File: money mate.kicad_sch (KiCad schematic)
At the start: 17 parts, among them SW1 SW_Push, SW2 SW_Push, SW3 SW_Push, SW4 RotaryEncoder_Switch, U1 MOUDLE-SEEEDUINO-XIAO

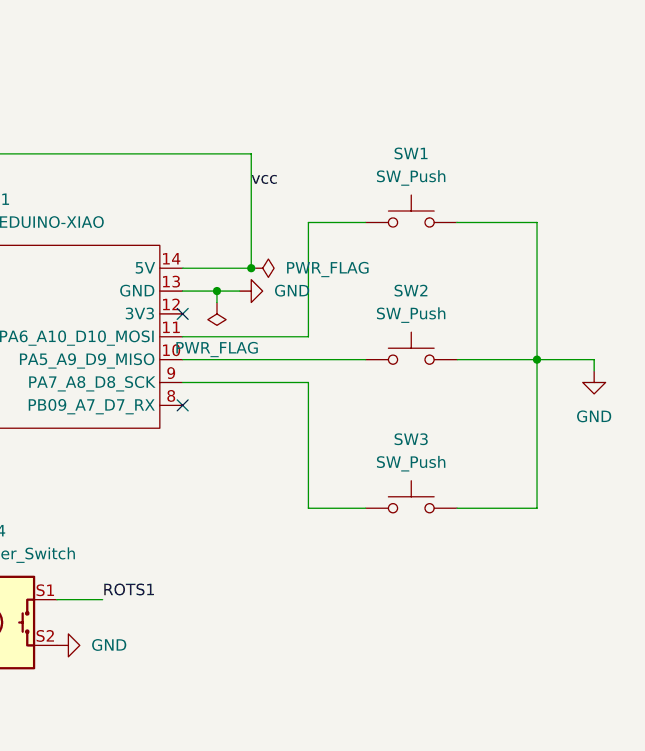
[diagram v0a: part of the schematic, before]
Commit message: pcb ready!!!!
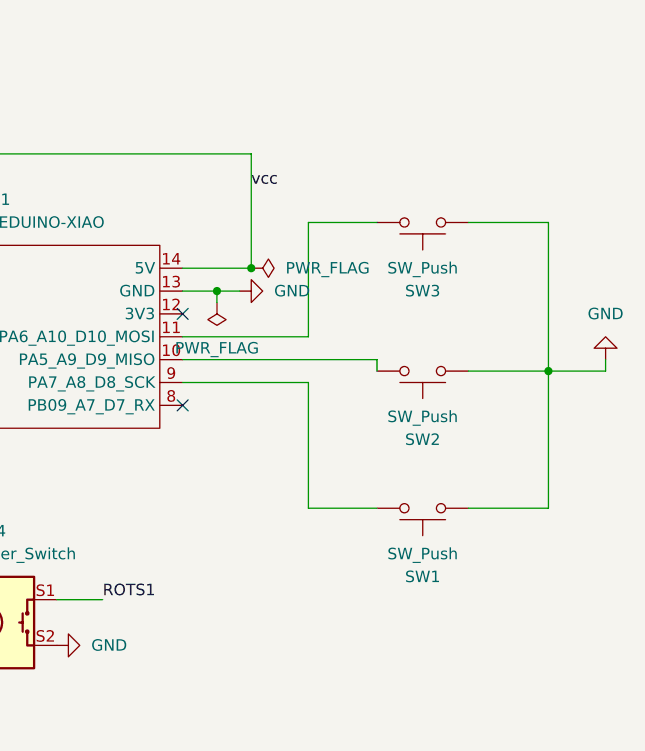
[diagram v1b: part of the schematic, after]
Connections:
- net at SW3.1: now also U1.11 (PA6_A10_D10_MOSI); no longer U1.9 (PA7_A8_D8_SCK)
- net at SW1.1: now also U1.9 (PA7_A8_D8_SCK); no longer U1.11 (PA6_A10_D10_MOSI)
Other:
- moved on the sheet: SW1, SW2, SW3
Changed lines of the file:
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@@
 	)
 	(junction
-		(at 233.68 86.36)
+		(at 234.95 87.63)
 		(diameter 0)
 		(color 0 0 0 0)
@@
 	(wire
 		(pts
+			(xy 215.9 87.63) (xy 215.9 86.36)
+		)
+		(stroke
+			(width 0)
+			(type default)
+		)
+	)
+	(wire
+		(pts
 			(xy 138.43 86.36) (xy 153.67 86.36)
 		)
@@
 	(wire
 		(pts
-			(xy 233.68 86.36) (xy 233.68 102.87)
+			(xy 234.95 87.63) (xy 234.95 71.12)
 		)
 		(stroke
@@
 	(wire
 		(pts
-			(xy 233.68 71.12) (xy 233.68 86.36)
+			(xy 234.95 102.87) (xy 234.95 87.63)
 		)
 		(stroke
@@
 	(wire
 		(pts
-			(xy 240.03 86.36) (xy 240.03 87.63)
+			(xy 241.3 87.63) (xy 241.3 86.36)
 		)
 		(stroke
@@
 	(wire
 		(pts
-			(xy 224.79 71.12) (xy 233.68 71.12)
+			(xy 226.06 102.87) (xy 234.95 102.87)
 		)
 		(stroke
@@
 	(wire
 		(pts
-			(xy 224.79 86.36) (xy 233.68 86.36)
+			(xy 226.06 87.63) (xy 234.95 87.63)
 		)
 		(stroke
@@
 	(wire
 		(pts
-			(xy 208.28 71.12) (xy 214.63 71.12)
+			(xy 208.28 71.12) (xy 215.9 71.12)
 		)
 		(stroke
@@
 	(wire
 		(pts
-			(xy 233.68 102.87) (xy 224.79 102.87)
+			(xy 234.95 71.12) (xy 226.06 71.12)
 		)
 		(stroke
@@
 	(wire
 		(pts
-			(xy 194.31 86.36) (xy 214.63 86.36)
+			(xy 194.31 86.36) (xy 215.9 86.36)
 		)
 		(stroke
@@
 	(wire
 		(pts
-			(xy 233.68 86.36) (xy 240.03 86.36)
+			(xy 234.95 87.63) (xy 241.3 87.63)
 		)
 		(stroke
@@
 	(wire
 		(pts
-			(xy 208.28 102.87) (xy 214.63 102.87)
+			(xy 208.28 102.87) (xy 215.9 102.87)
 		)
 		(stroke
@@
 	(symbol
 		(lib_id "power:GND")
-		(at 240.03 87.63 0)
+		(at 241.3 86.36 0)
+		(mirror x)
 		(unit 1)
 		(body_style 1)
@@
 		(fields_autoplaced yes)
 		(property "Reference" "#PWR02"
-			(at 240.03 93.98 0)
+			(at 241.3 80.01 0)
 			(hide yes)
 			(show_name no)
@@
 		)
 		(property "Value" "GND"
-			(at 240.03 92.71 0)
+			(at 241.3 81.28 0)
 			(show_name no)
 			(do_not_autoplace no)
@@
 		)
 		(property "Footprint" ""
-			(at 240.03 87.63 0)
+			(at 241.3 86.36 0)
 			(hide yes)
 			(show_name no)
@@
 		)
 		(property "Datasheet" ""
-			(at 240.03 87.63 0)
+			(at 241.3 86.36 0)
 			(hide yes)
 			(show_name no)
@@
 		)
 		(property "Description" "Power symbol creates a global label with name \"GND\" , ground"
-			(at 240.03 87.63 0)
+			(at 241.3 86.36 0)
 			(hide yes)
 			(show_name no)
@@
 	(symbol
 		(lib_id "Switch:SW_Push")
-		(at 219.71 102.87 0)
+		(at 220.98 71.12 0)
+		(mirror x)
 		(unit 1)
 		(body_style 1)
@@
 		(fields_autoplaced yes)
 		(property "Reference" "SW3"
-			(at 219.71 95.25 0)
+			(at 220.98 78.74 0)
 			(show_name no)
 			(do_not_autoplace no)
@@
 		)
 		(property "Value" "SW_Push"
-			(at 219.71 97.79 0)
+			(at 220.98 76.2 0)
 			(show_name no)
 			(do_not_autoplace no)
@@
 		)
 		(property "Footprint" "Button_Switch_Keyboard:SW_Cherry_MX_1.00u_PCB"
-			(at 219.71 97.79 0)
+			(at 220.98 76.2 0)
 			(hide yes)
 			(show_name no)
@@
 		)
 		(property "Datasheet" ""
-			(at 219.71 97.79 0)
+			(at 220.98 76.2 0)
 			(hide yes)
 			(show_name no)
@@
 		)
 		(property "Description" "Push button switch, generic, two pins"
-			(at 219.71 102.87 0)
+			(at 220.98 71.12 0)
 			(hide yes)
 			(show_name no)
@@
 	(symbol
 		(lib_id "Switch:SW_Push")
-		(at 219.71 71.12 0)
+		(at 220.98 102.87 0)
+		(mirror x)
 		(unit 1)
 		(body_style 1)
@@
 		(fields_autoplaced yes)
 		(property "Reference" "SW1"
-			(at 219.71 63.5 0)
+			(at 220.98 110.49 0)
 			(show_name no)
 			(do_not_autoplace no)
@@
 		)
 		(property "Value" "SW_Push"
-			(at 219.71 66.04 0)
+			(at 220.98 107.95 0)
 			(show_name no)
 			(do_not_autoplace no)
@@
 		)
 		(property "Footprint" "Button_Switch_Keyboard:SW_Cherry_MX_1.00u_PCB"
-			(at 219.71 66.04 0)
+			(at 220.98 107.95 0)
 			(hide yes)
 			(show_name no)
@@
 		)
 		(property "Datasheet" ""
-			(at 219.71 66.04 0)
+			(at 220.98 107.95 0)
 			(hide yes)
 			(show_name no)
@@
 		)
 		(property "Description" "Push button switch, generic, two pins"
-			(at 219.71 71.12 0)
+			(at 220.98 102.87 0)
 			(hide yes)
 			(show_name no)
@@
 	(symbol
 		(lib_id "Switch:SW_Push")
-		(at 219.71 86.36 0)
+		(at 220.98 87.63 0)
+		(mirror x)
 		(unit 1)
 		(body_style 1)
@@
 		(fields_autoplaced yes)
 		(property "Reference" "SW2"
-			(at 219.71 78.74 0)
+			(at 220.98 95.25 0)
 			(show_name no)
 			(do_not_autoplace no)
@@
 		)
 		(property "Value" "SW_Push"
-			(at 219.71 81.28 0)
+			(at 220.98 92.71 0)
 			(show_name no)
 			(do_not_autoplace no)
@@
 		)
 		(property "Footprint" "Button_Switch_Keyboard:SW_Cherry_MX_1.00u_PCB"
-			(at 219.71 81.28 0)
+			(at 220.98 92.71 0)
 			(hide yes)
 			(show_name no)
@@
 		)
 		(property "Datasheet" ""
-			(at 219.71 81.28 0)
+			(at 220.98 92.71 0)
 			(hide yes)
 			(show_name no)
@@
 		)
 		(property "Description" "Push button switch, generic, two pins"
-			(at 219.71 86.36 0)
+			(at 220.98 87.63 0)
 			(hide yes)
 			(show_name no)
